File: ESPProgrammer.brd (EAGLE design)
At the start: 31.4 x 40.6 mm, 3 parts

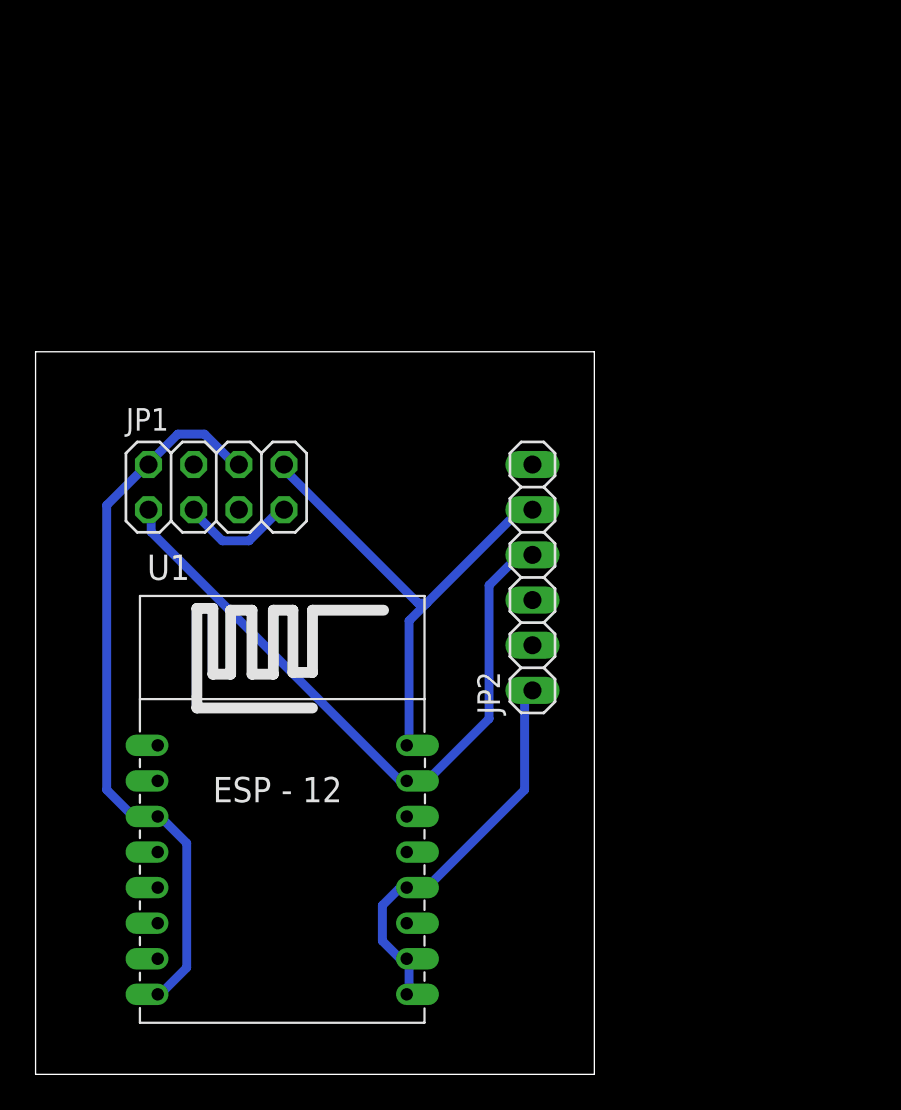
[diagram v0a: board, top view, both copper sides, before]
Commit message: update file
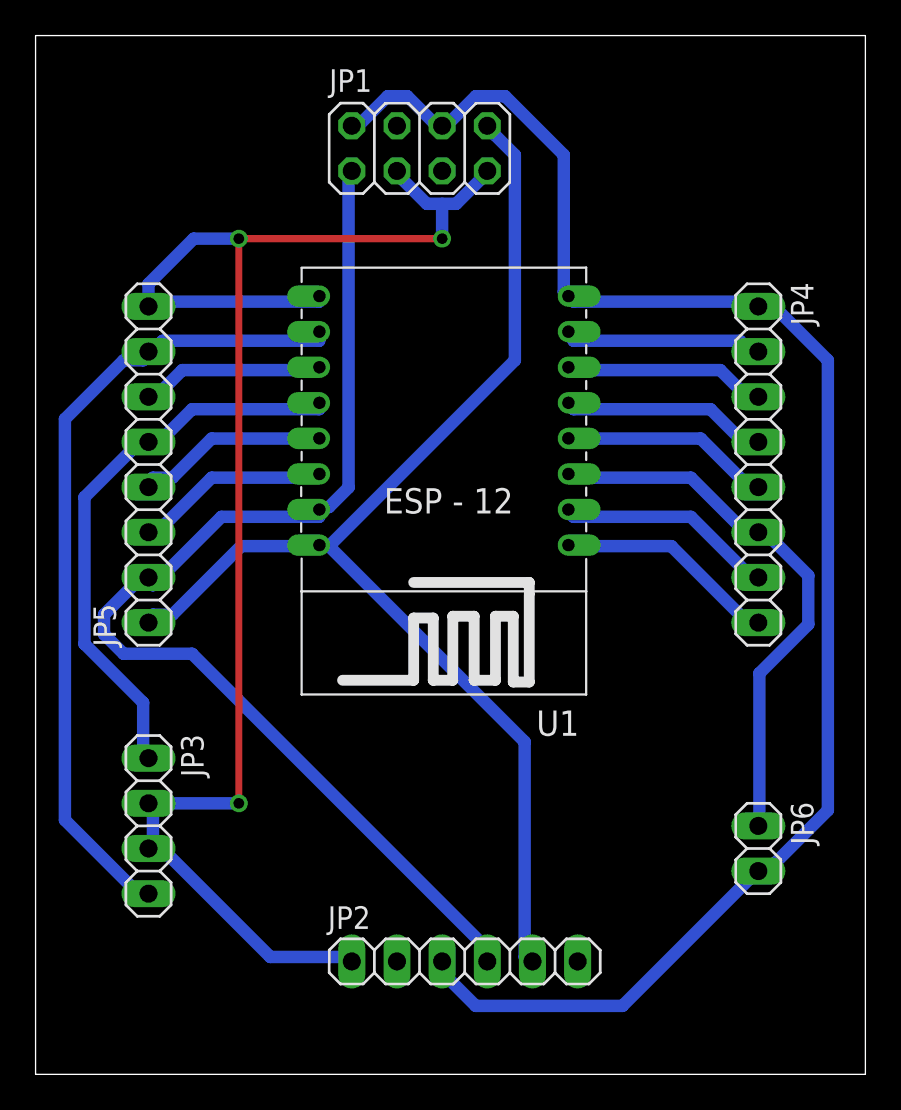
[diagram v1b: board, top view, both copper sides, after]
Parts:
- added JP3: (no value), pinhead:1X04
- added JP4, JP5: (no value), pinhead:1X08
- added JP6: (no value), pinhead:1X02
- moved U1 24.5 mm to (22.9, 35.6), turned to 180 degrees
- moved JP1 22.2 mm to (21.6, 52.1)
- moved JP2 21.9 mm to (24.1, 6.35), turned to 0 degrees
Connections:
- new net N$1: JP3.1, JP5.5, U1.GPIO0
- new net N$10: JP4.7, U1.ADC
- new net N$11: JP4.5, U1.GPIO16
- new net N$12: JP4.4, U1.GPIO14
- new net N$13: JP4.3, U1.GPIO12
- new net N$14: JP4.2, U1.GPIO13
- new net N$15: JP4.6, JP6.1, U1.CH_PD
- new net N$2: JP3.4, JP5.7, U1.GPIO15
- new net N$3: JP5.3, U1.GPIO4
- new net N$6: JP5.4, U1.GPIO5
- new net N$7: JP5.6, U1.GPIO2
- new net N$9: JP4.8, U1.RESET
- net GND: now also JP3.2, JP3.3, JP5.8; no longer U1.GPIO0, U1.GPIO15
- net N$4: now also JP5.2
- net N$5: now also JP5.1
- net VCC: now also JP4.1, JP6.2; no longer U1.CH_PD
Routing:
- net GND: track 29.2 -> 92.0 mm, vias 0 -> 3
- net VCC: track 40.8 -> 92.5 mm
- net N$2: track 0.00 -> 45.6 mm
- net N$5: track 28.2 -> 68.8 mm
- net N$1: track 0.00 -> 32.2 mm
- net N$15: track 0.00 -> 31.6 mm
- net N$4: track 38.4 -> 65.9 mm
- net N$9: track 0.00 -> 12.5 mm
- net N$10: track 0.00 -> 12.3 mm
- net N$12: track 0.00 -> 11.9 mm
- net N$11: track 0.00 -> 11.8 mm
- net N$13: track 0.00 -> 11.4 mm
- net N$3: track 0.00 -> 11.3 mm
- net N$14: track 0.00 -> 11.2 mm
- net N$6: track 0.00 -> 10.9 mm
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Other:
- board size 31.4 x 40.6 mm -> 46.7 x 58.4 mm
